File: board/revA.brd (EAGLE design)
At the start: 50 x 50 mm, 56 parts, among them IC1 74HCT125, Q1 VND7NV04, Q2 VND7NV04, Q3 VND7NV04, Q4 VND7NV04

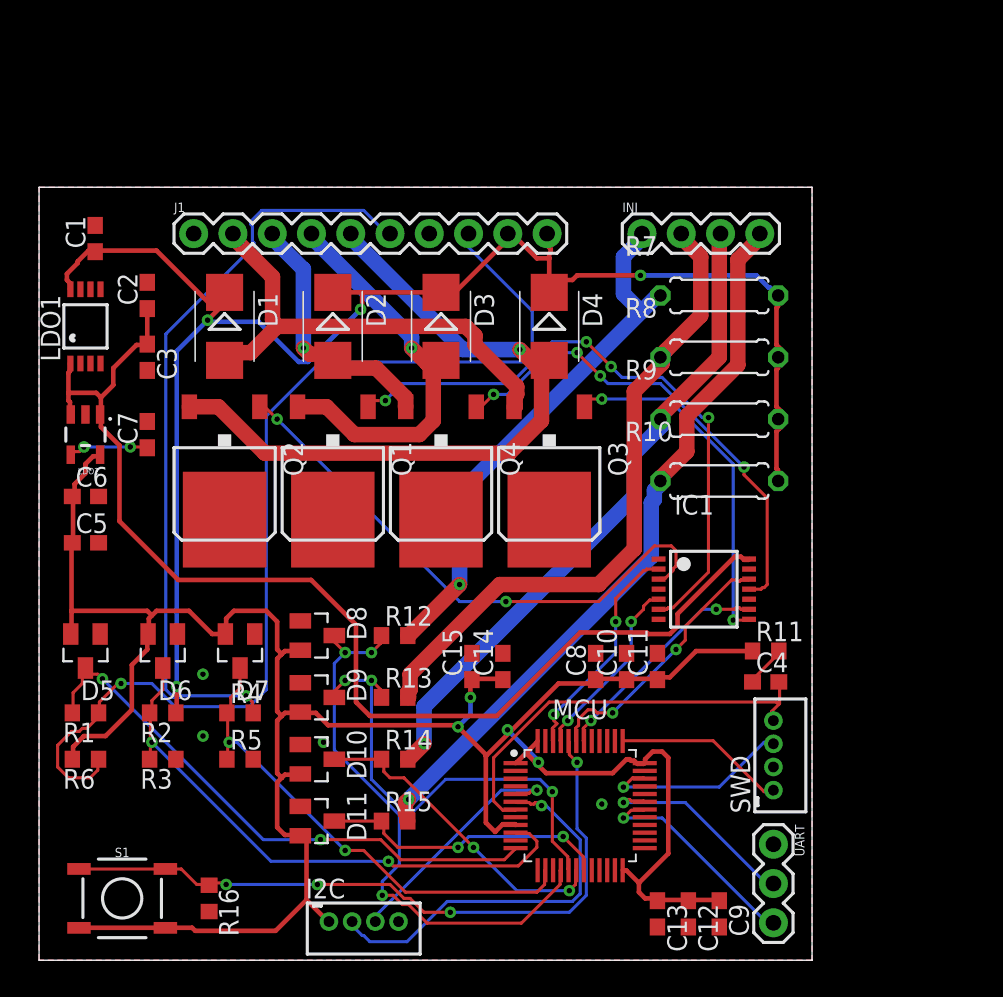
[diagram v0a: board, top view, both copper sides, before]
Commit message: More routing tests
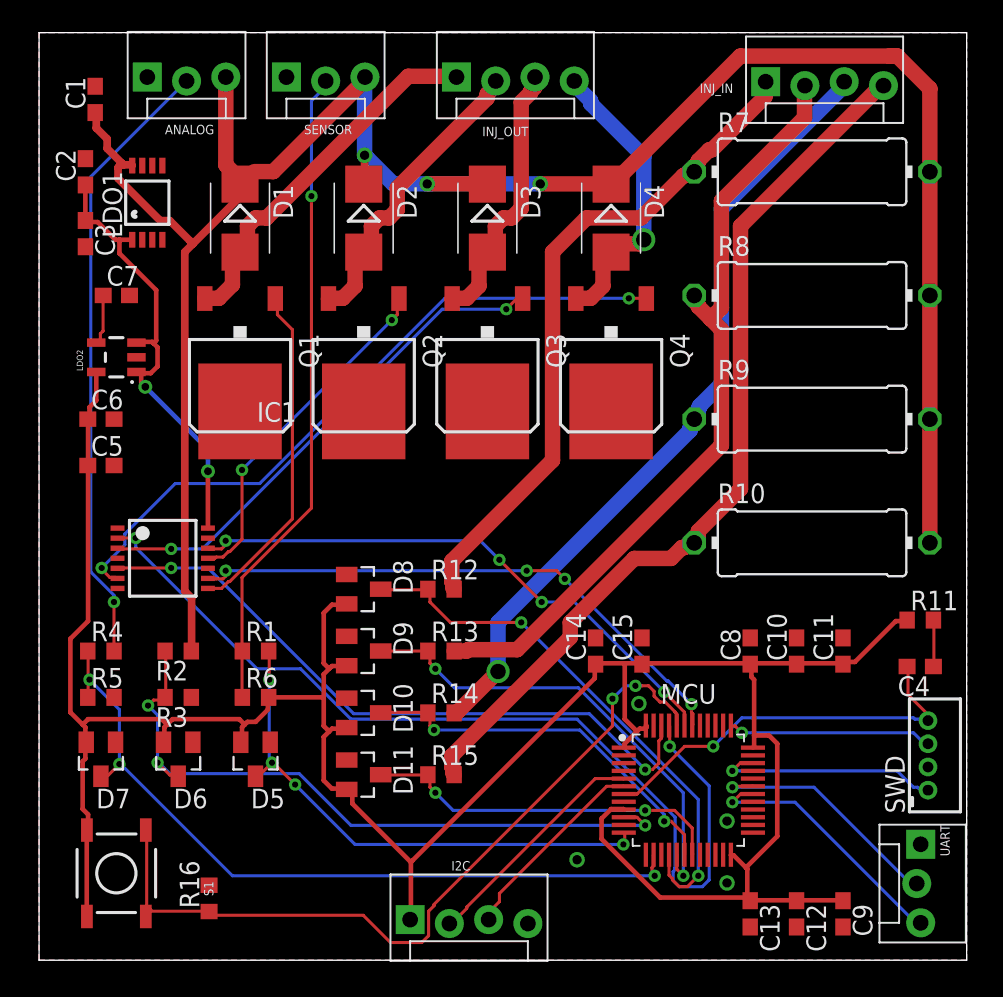
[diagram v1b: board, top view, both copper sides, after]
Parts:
- removed INJ: (no value), SparkFun-Connectors:1X04
- removed J1: (no value), SparkFun-Connectors:1X10
- added ANALOG, SENSOR: (no value), SparkFun-Connectors:MOLEX-1X3_LOCK
- added INJ_IN, INJ_OUT: (no value), SparkFun-Connectors:MOLEX-1X4_LOCK
- I2C: value B4B-ZR -> (none); device con-jst:B4B-ZR -> SparkFun-Connectors:MOLEX-1X4_LOCK
- R10, R7, R8, R9: device rcl:0207/7 -> rcl:0414/15
- UART: device SparkFun-Connectors:1X03 -> SparkFun-Connectors:MOLEX-1X3_LOCK
- moved IC1 35.1 mm to (8.00, 26.0)
- moved D5 13.0 mm to (14.0, 13.0)
- moved Q4 13.0 mm to (37.0, 38.0)
- moved C11 12.0 mm to (52.0, 20.0)
- moved R1 11.7 mm to (14.0, 20.0), turned to 0 degrees
- moved R6 11.7 mm to (14.0, 17.0), turned to 0 degrees
- moved D7 11.4 mm to (4.00, 13.0)
- moved Q2 11.4 mm to (21.0, 38.0)
- moved C10 11.0 mm to (49.0, 20.0)
- moved C15 11.0 mm to (39.0, 20.0)
- moved R11 10.2 mm to (57.0, 22.0)
- moved C4 10.0 mm to (57.0, 19.0), turned to 180 degrees
- moved C8 10.0 mm to (46.0, 20.0)
- moved R7 10.0 mm to (50.0, 51.0)
- moved SWD 10.0 mm to (57.5, 13.2)
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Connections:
- net N$5 renamed BUTTON
- net AN1: now also ANALOG.2; no longer J1.6
- net FF_SIG: now also SENSOR.2; no longer J1.8
- net GND: now also ANALOG.1, SENSOR.1; no longer J1.1, J1.7
- net I2C_SCL: now also I2C.3; no longer I2C.2
- net I2C_SDA: now also I2C.2; no longer I2C.3
- net INJ1: now also INJ_OUT.1, Q1.3; no longer J1.2, Q3.3
- net INJ1_IN: now also INJ_IN.1; no longer INJ.1
- net INJ2: now also INJ_OUT.2, Q2.3; no longer J1.3, Q4.3
- net INJ2_IN: now also INJ_IN.2; no longer INJ.2
- net INJ3: now also INJ_OUT.3, Q3.3; no longer J1.4, Q1.3
- net INJ3_IN: now also INJ_IN.3; no longer INJ.3
- net INJ3_TRIGGER: now also IC1.2; no longer IC1.5
- net INJ4: now also INJ_OUT.4, Q4.3; no longer J1.5, Q2.3
- net INJ4_IN: now also INJ_IN.4; no longer INJ.4
- net INJ4_TRIGGER: now also IC1.5; no longer IC1.2
- net N$10: now also IC1.3; no longer IC1.8
- net N$7: now also IC1.11; no longer IC1.3
- net N$8: now also IC1.8; no longer IC1.6
- net N$9: now also IC1.6; no longer IC1.11
- net SWCLK: now also SWD.3; no longer SWD.1
- net SWDIO: now also SWD.1; no longer SWD.3
- net VCC: now also ANALOG.3, SENSOR.3; no longer J1.10, J1.9
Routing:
- net INJ3_TRIGGER: track 12.1 -> 61.9 mm
- net +5V: track 75.4 -> 30.1 mm, vias 0 -> 2
- net VCC: track 105.6 -> 145.7 mm, vias 4 -> 3
- net INJ4_TRIGGER: track 14.7 -> 43.2 mm
- net INJ4: track 45.6 -> 19.1 mm
- net FF_SIG: track 68.1 -> 42.2 mm
- net INJ1_TRIGGER: track 14.9 -> 36.7 mm, vias 2 -> 4
- net INJ2_TRIGGER: track 17.1 -> 36.7 mm, vias 2 -> 4
- net AN_1: track 32.0 -> 50.0 mm, vias 2 -> 3
- net N$8: track 40.0 -> 22.0 mm, vias 4 -> 0
- net N$7: track 36.3 -> 22.5 mm
- net N$9: track 31.4 -> 44.2 mm, vias 4 -> 2
- net I2C_SCL: track 25.5 -> 13.0 mm, vias 1 -> 0
- net INJ4_IN: track 47.6 -> 58.2 mm, vias 1 -> 0
- net N$10: track 22.9 -> 33.0 mm
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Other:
- board size 50 x 50 mm -> 60 x 60 mm
